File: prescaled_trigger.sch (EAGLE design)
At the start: 27 parts, among them X1 BU-SMA-H, X2 BU-SMA-H, X3 BU-SMA-H

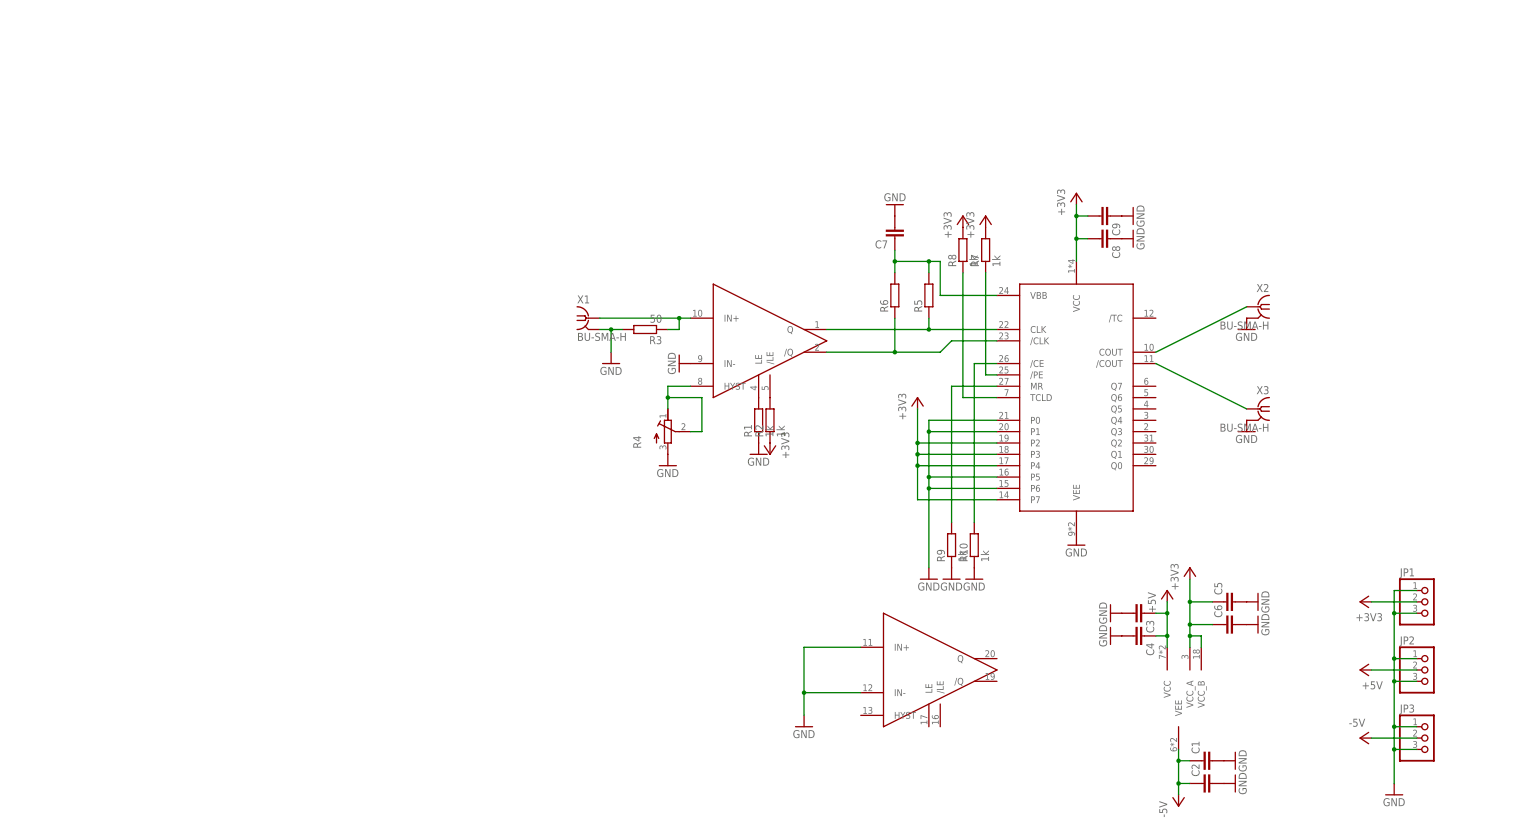
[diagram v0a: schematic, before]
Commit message: tracking board layout
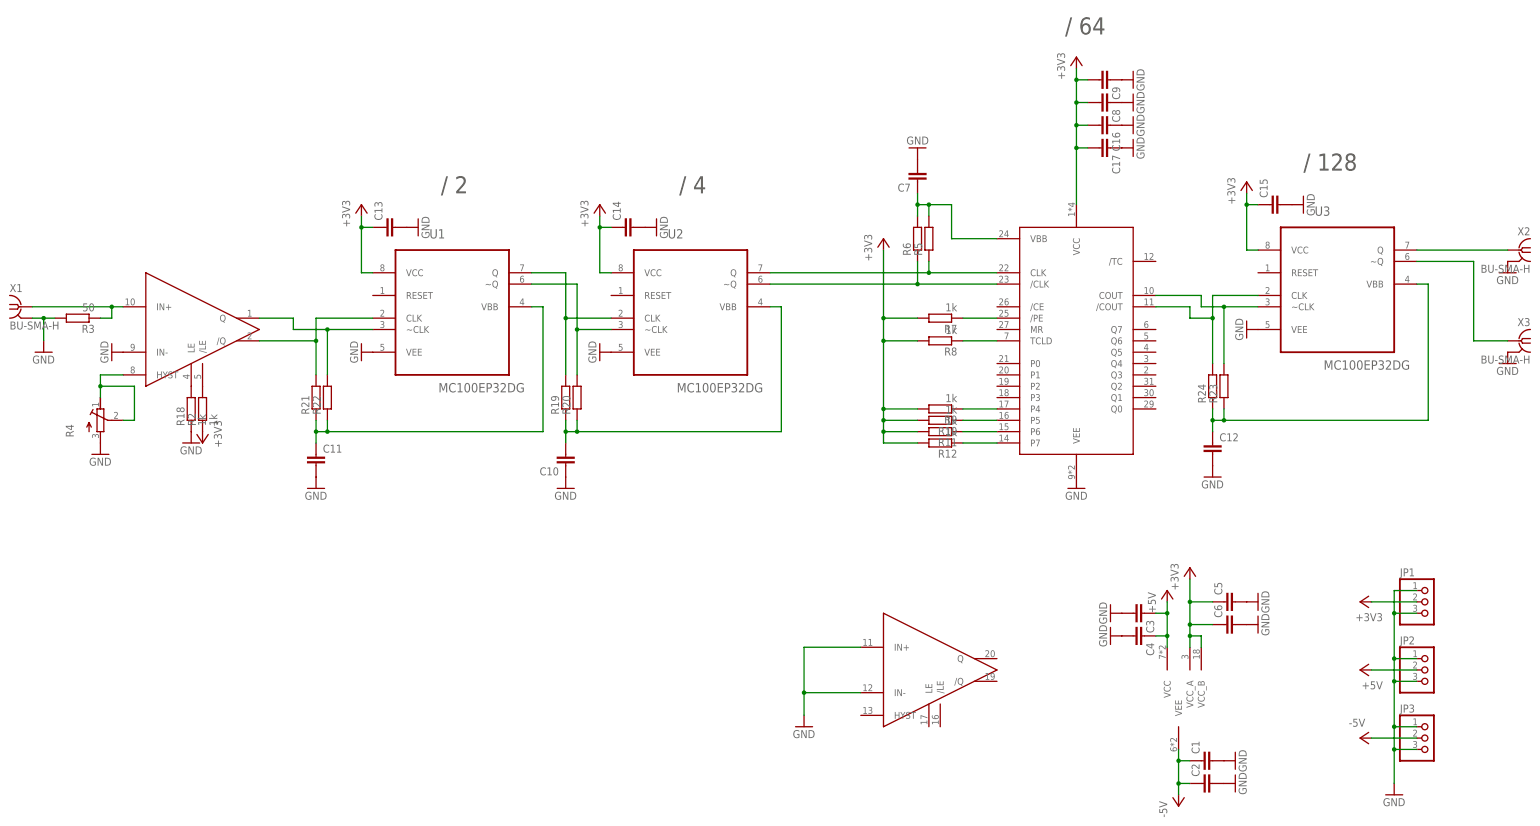
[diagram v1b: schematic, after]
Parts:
- removed R1: 1k, resistor:R-EU_M0805
- added C10, C11, C12, C13, C14, C15, C16, C17: (no value), resistor:C-EUC0805
- added R11, R12, R18: 1k, resistor:R-EU_M0805
- added R19, R20, R21, R22, R23, R24: (no value), resistor:R-EU_M1206
- added U1, U2, U3: MC100EP32DG, MC100EP32:MC100EP32DG
- R5, R6: device resistor:R-EU_M0805 -> resistor:R-EU_M1206
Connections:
- removed net /TRIGOUT: U$2./COUT, X3.1
- removed net N$1: R1.2, U$1G$1.LE
- removed net N$12: R9.2, U$2.MR
- removed net N$13: R10.2, U$2./CE
- removed net TRIGOUT: U$2.COUT, X2.1
- new net N$15: R18.2, U$1G$1.LE
- new net N$16: C11.1, R21.1, R22.1, U1.VBB
- new net N$17: R21.2, U$1G$1./Q, U1.CLK
- new net N$18: R22.2, U$1G$1.Q, U1.~CLK
- new net N$19: C10.2, R19.1, R20.1, U2.VBB
- new net N$20: R19.2, U1.Q, U2.CLK
- new net N$21: R20.2, U1.~Q, U2.~CLK
- new net N$26: U3.Q, X2.1
- new net N$27: U3.~Q, X3.1
- new net N$28: C12.1, R23.1, R24.1, U3.VBB
- new net N$29: R24.2, U$2./COUT, U3.CLK
- new net N$3: R11.1, U$2.P6
- new net N$30: R23.2, U$2.COUT, U3.~CLK
- new net N$5: R10.1, U$2.P5
- new net N$6: R9.1, U$2.P4
- new net N$7: R12.1, U$2.P7
- net +3V3: now also C13.1, C14.1, C15.1, C16.2, C17.2, R10.2, R11.2, R12.2, R9.2, U1.VCC, U2.VCC, U3.VCC; no longer U$2.P2, U$2.P3, U$2.P4, U$2.P7
- net /CLKIN: now also U2.~Q; no longer U$1G$1./Q
- net CLKIN: now also U2.Q; no longer U$1G$1.Q
- net GND: now also C10.1, C11.2, C12.2, C13.2, C14.2, C15.2, C16.1, C17.1, R18.1, U1.VEE, U2.VEE, U3.VEE; no longer R1.1, R10.1, R9.1, U$2.P0, U$2.P1, U$2.P5, U$2.P6
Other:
- note added: "/ 128"
- note added: "/ 2"
- note added: "/ 4"
- note added: "/ 64"
- moved on the sheet: C7, C8, C9, R10, R2, R3, R4, R5, R6, R7, R8, R9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
